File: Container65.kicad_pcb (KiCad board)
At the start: 2 copper layers, 81 x 99.2 mm, 90 parts, among them J1 Conn_01x03, J2 Conn_01x06, U1 RP2040, U2 TYPE-C-31-M-12, U3 XC6206PxxxMR, U4 W25Q128JVS, U5 USB Boot, U6 Reset, U7 LEFT, U8 RIGHT, Y1 12MHz - 20pF

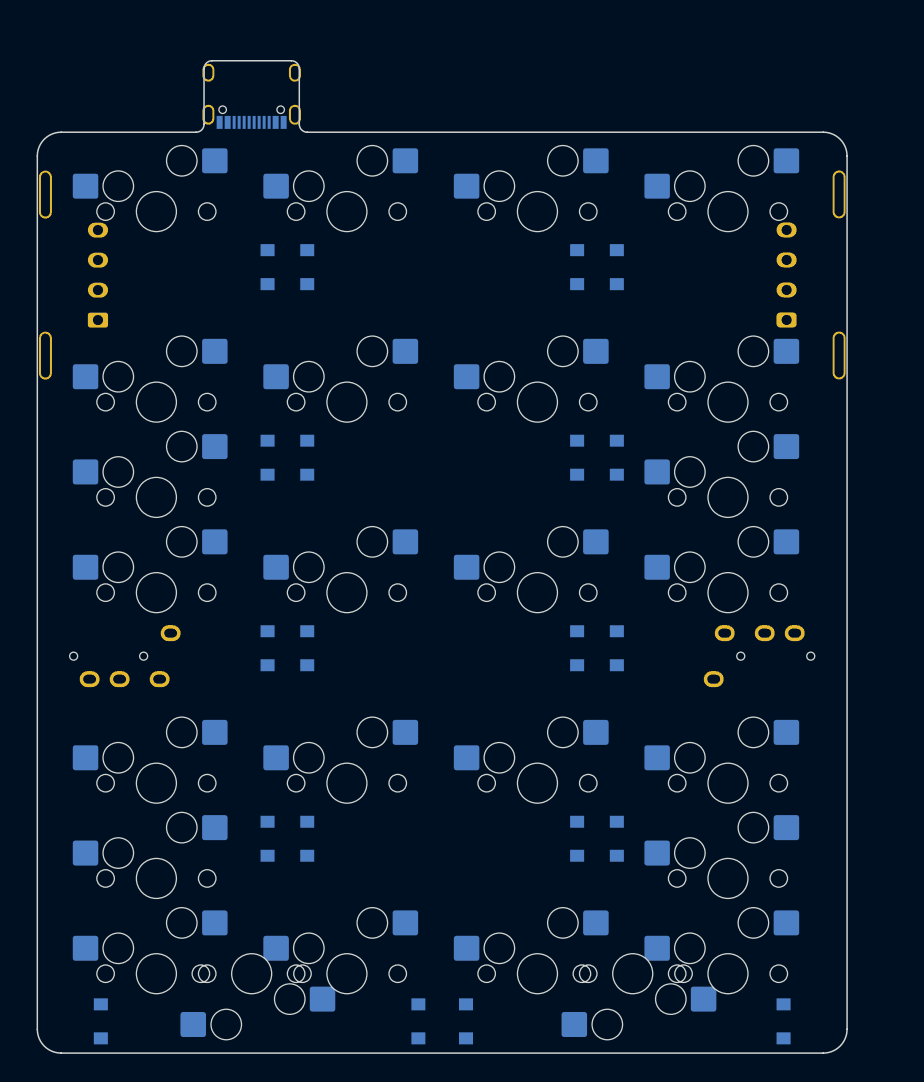
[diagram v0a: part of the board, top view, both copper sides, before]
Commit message: Copy from backup
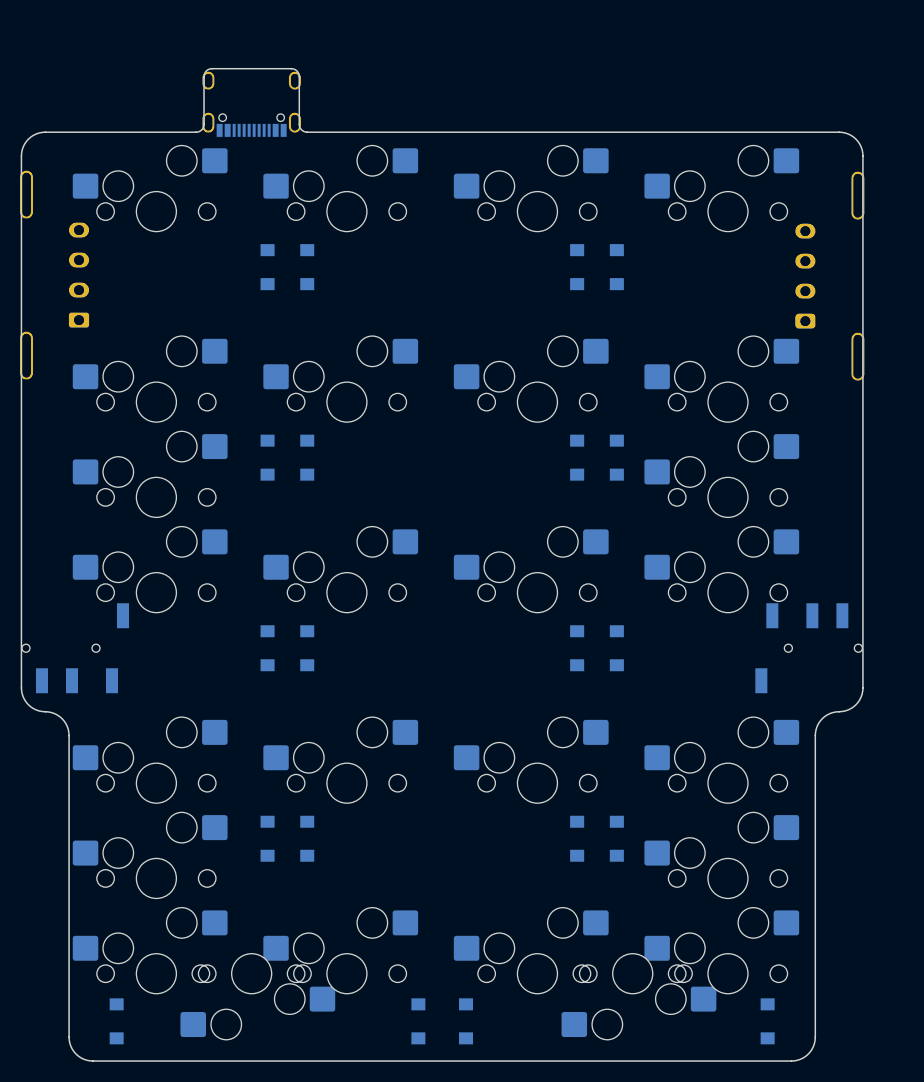
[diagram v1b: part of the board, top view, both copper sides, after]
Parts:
- U7, U8: footprint Keebio-Parts:TRRS-PJ-320A -> Keebio-Parts:TRRS-PJ-320D
- moved U8 4.83 mm to (121.0, 92.1)
- moved U7 4.83 mm to (34.6, 92.1)
- moved POGO1 1.89 mm to (41.5, 54.8)
- moved POGO2 1.88 mm to (114.1, 54.9)
- moved D20 1.59 mm to (110.3, 129.4)
- moved D17 1.59 mm to (45.2, 129.4)
- moved U2 0.79 mm to (58.7, 36.5)
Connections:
- U7 pad 1: unconnected-(U7-Pad1) -> SCL
- U7 pad 2: unconnected-(U7-Pad2) -> VCC
- U7 pad 3: unconnected-(U7-Pad3) -> GND
- U7 pad 4: unconnected-(U7-Pad4) -> SDA
- U8 pad 1: unconnected-(U8-Pad1) -> SCL
- U8 pad 2: unconnected-(U8-Pad2) -> VCC
- U8 pad 3: unconnected-(U8-Pad3) -> GND
- U8 pad 4: unconnected-(U8-Pad4) -> SDA
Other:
- board size 81 x 99.2 mm -> 84.1 x 99.2 mm
